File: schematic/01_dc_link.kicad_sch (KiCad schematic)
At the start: 23 parts, among them J101 XT60PW-M, J102 MT60 / 12AWG pigtail, J103 CHASSIS

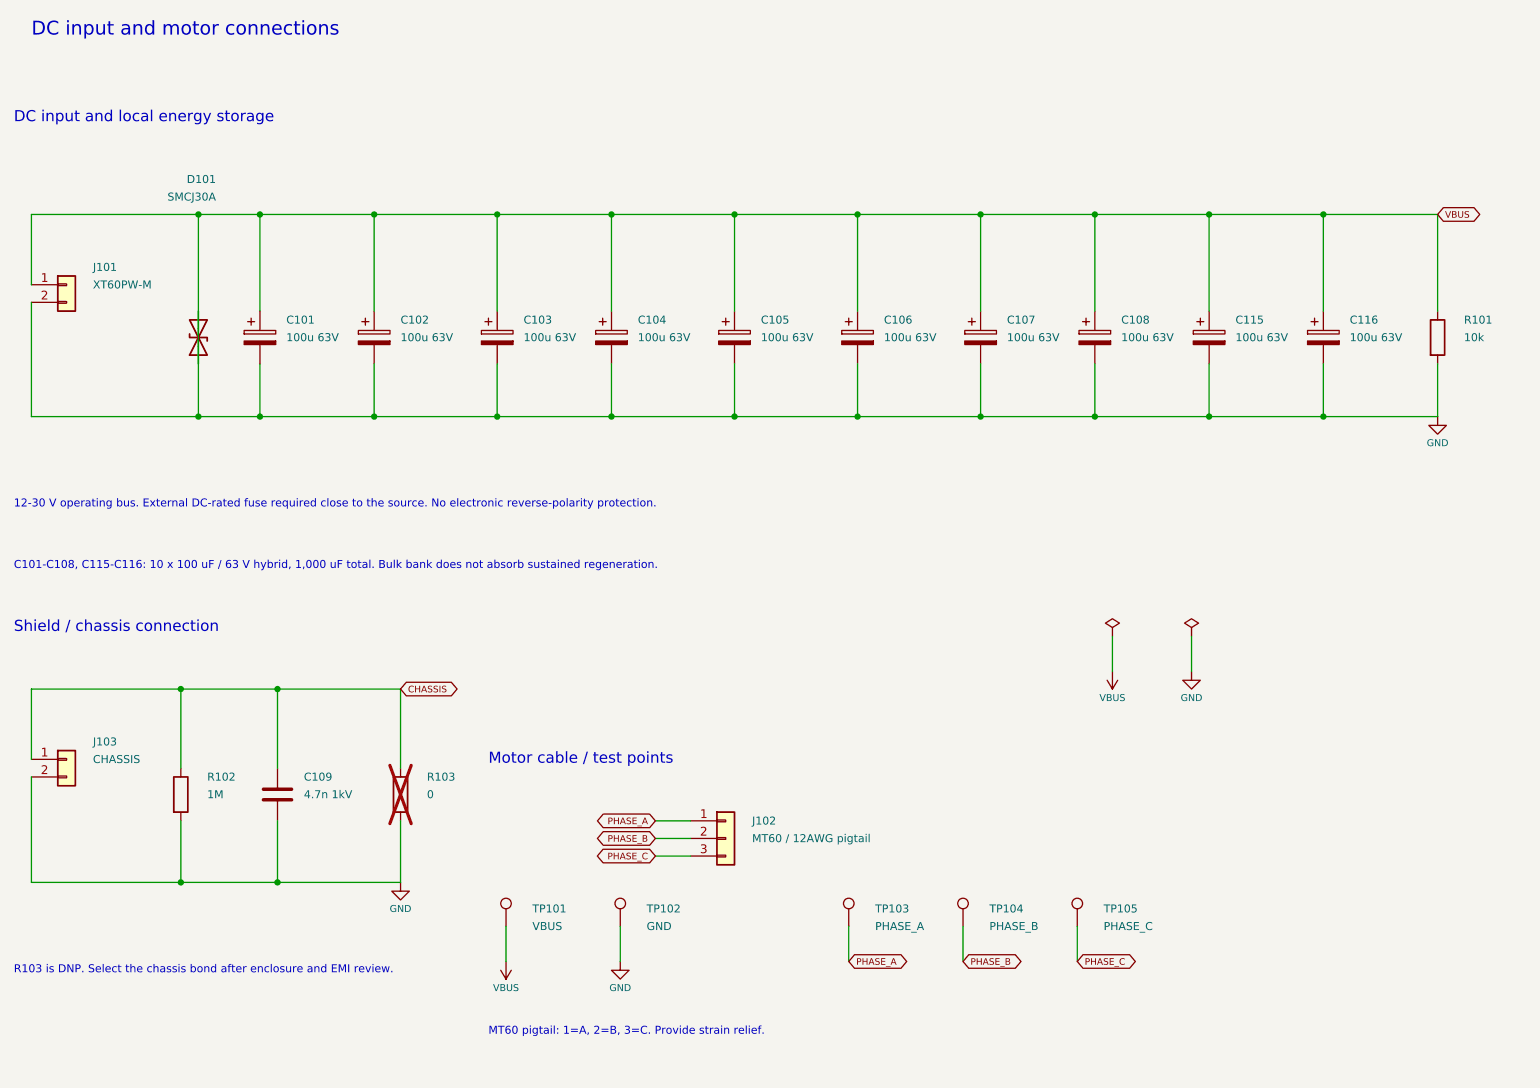
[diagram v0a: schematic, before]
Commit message: devlog 04
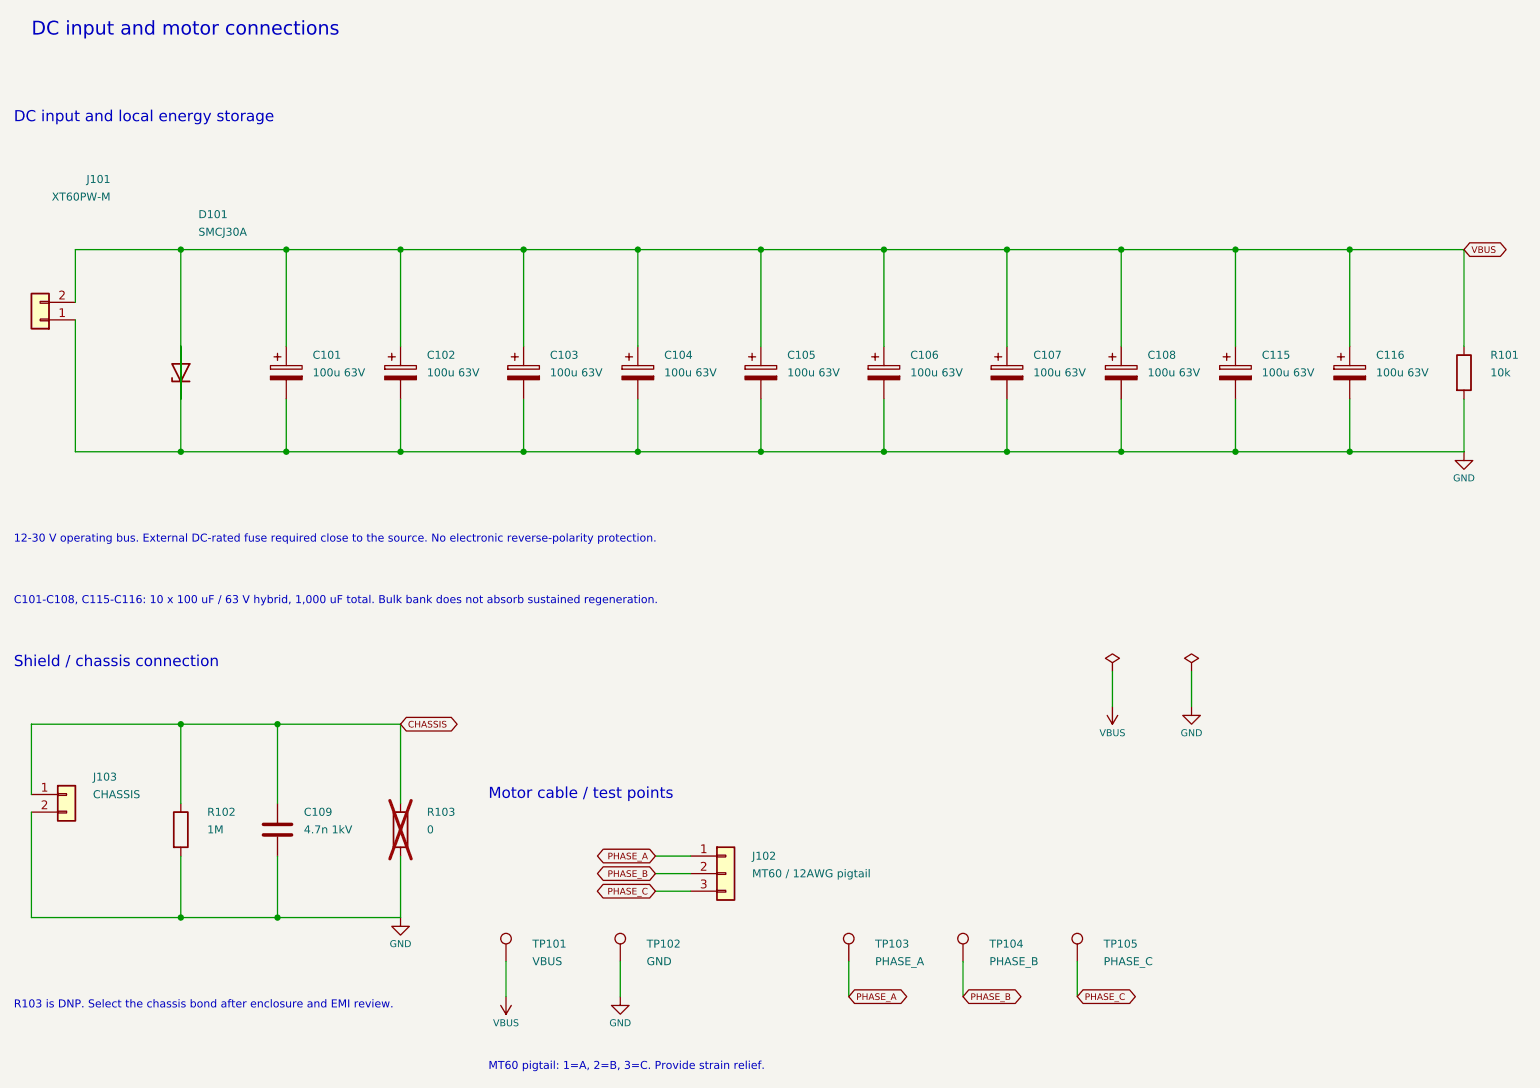
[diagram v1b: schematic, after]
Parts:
- C109: MPN C1206C472KGRACTU -> C1206C472KDRACTU; Manufacturer (none) -> KEMET
- D101: symbol Device:D_TVS -> Device:D_Zener; Manufacturer (none) -> Littelfuse
- J101, J102: Manufacturer (none) -> AMASS
- J103: Manufacturer (none) -> Harwin
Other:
- moved on the sheet: C101, C102, C103, C104, C105, C106, C107, C108, C109, C115, C116, D101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

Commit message: connect the bridge test points and snubbers
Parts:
- TP103, TP104, TP105: footprint TestPoint:TestPoint_Pad_D1.5mm -> bldc-esc:TestPoint_Pad_D1.5mm_NoSilk
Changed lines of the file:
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@@
       )
     )
-    (property "Footprint" "TestPoint:TestPoint_Pad_D1.5mm"
+    (property "Footprint" "bldc-esc:TestPoint_Pad_D1.5mm_NoSilk"
       (at 133.35 152.4 0)
       (effects
@@
       )
     )
-    (property "Footprint" "TestPoint:TestPoint_Pad_D1.5mm"
+    (property "Footprint" "bldc-esc:TestPoint_Pad_D1.5mm_NoSilk"
       (at 149.86 152.4 0)
       (effects
@@
       )
     )
-    (property "Footprint" "TestPoint:TestPoint_Pad_D1.5mm"
+    (property "Footprint" "bldc-esc:TestPoint_Pad_D1.5mm_NoSilk"
       (at 166.37 152.4 0)
       (effects

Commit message: add mounting holes and bring-up firmware
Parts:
- J101: footprint Connector_AMASS:AMASS_XT60PW-M_1x02_P7.20mm_Horizontal -> bldc-esc:XT60PW_M_Edge
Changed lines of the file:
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@@
       )
     )
-    (property "Footprint" "Connector_AMASS:AMASS_XT60PW-M_1x02_P7.20mm_Horizontal"
+    (property "Footprint" "bldc-esc:XT60PW_M_Edge"
       (at 16.51 59.69 0)
       (effects
